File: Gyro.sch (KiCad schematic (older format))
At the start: 7 parts, among them U5 SN74AXC4T774BQBR, U6 ICM-20948

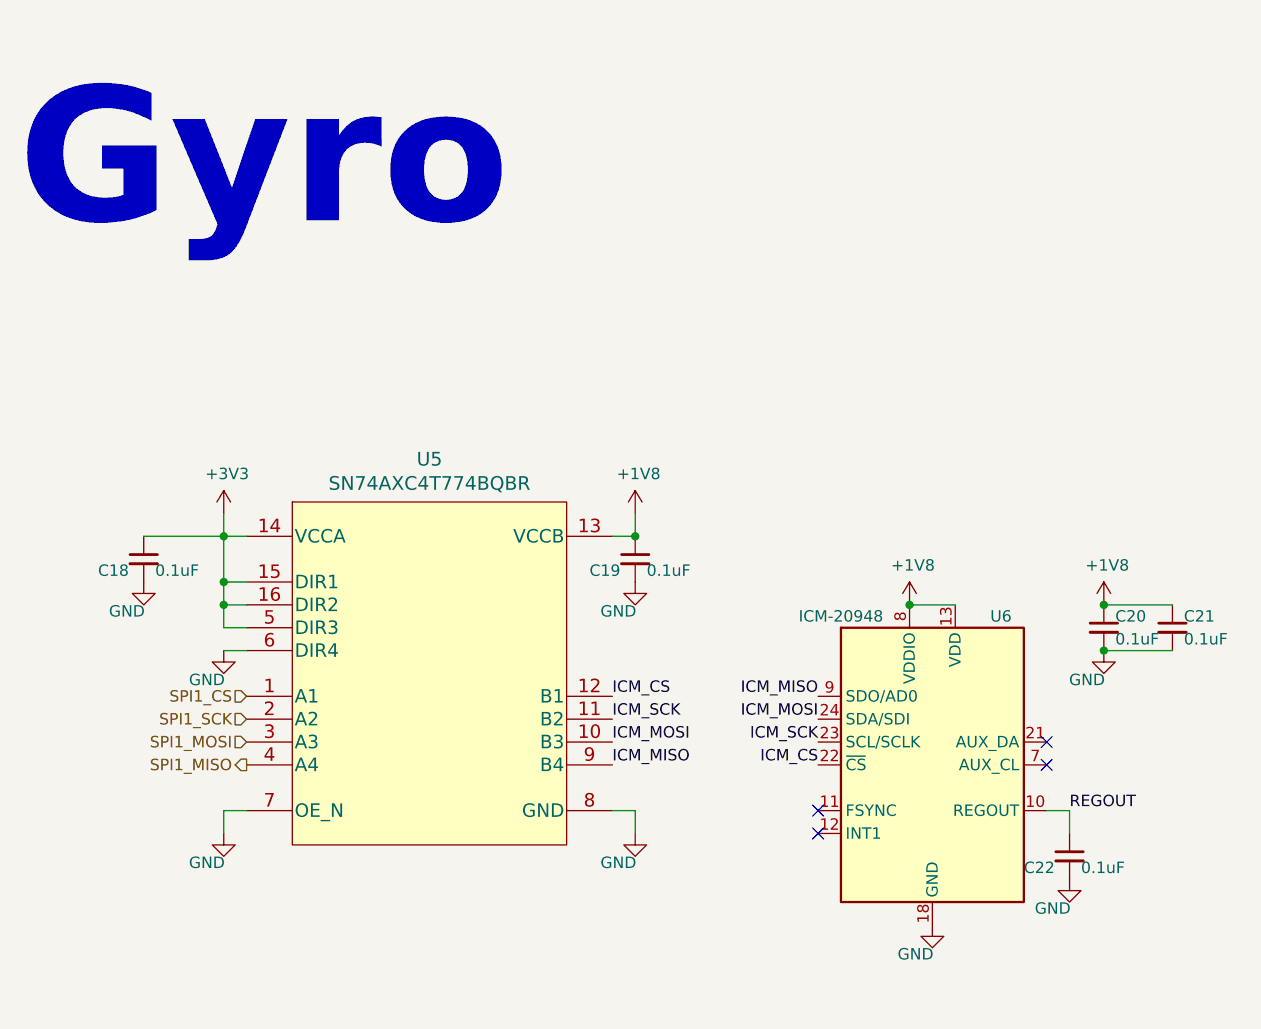
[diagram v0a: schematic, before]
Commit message: Changes made
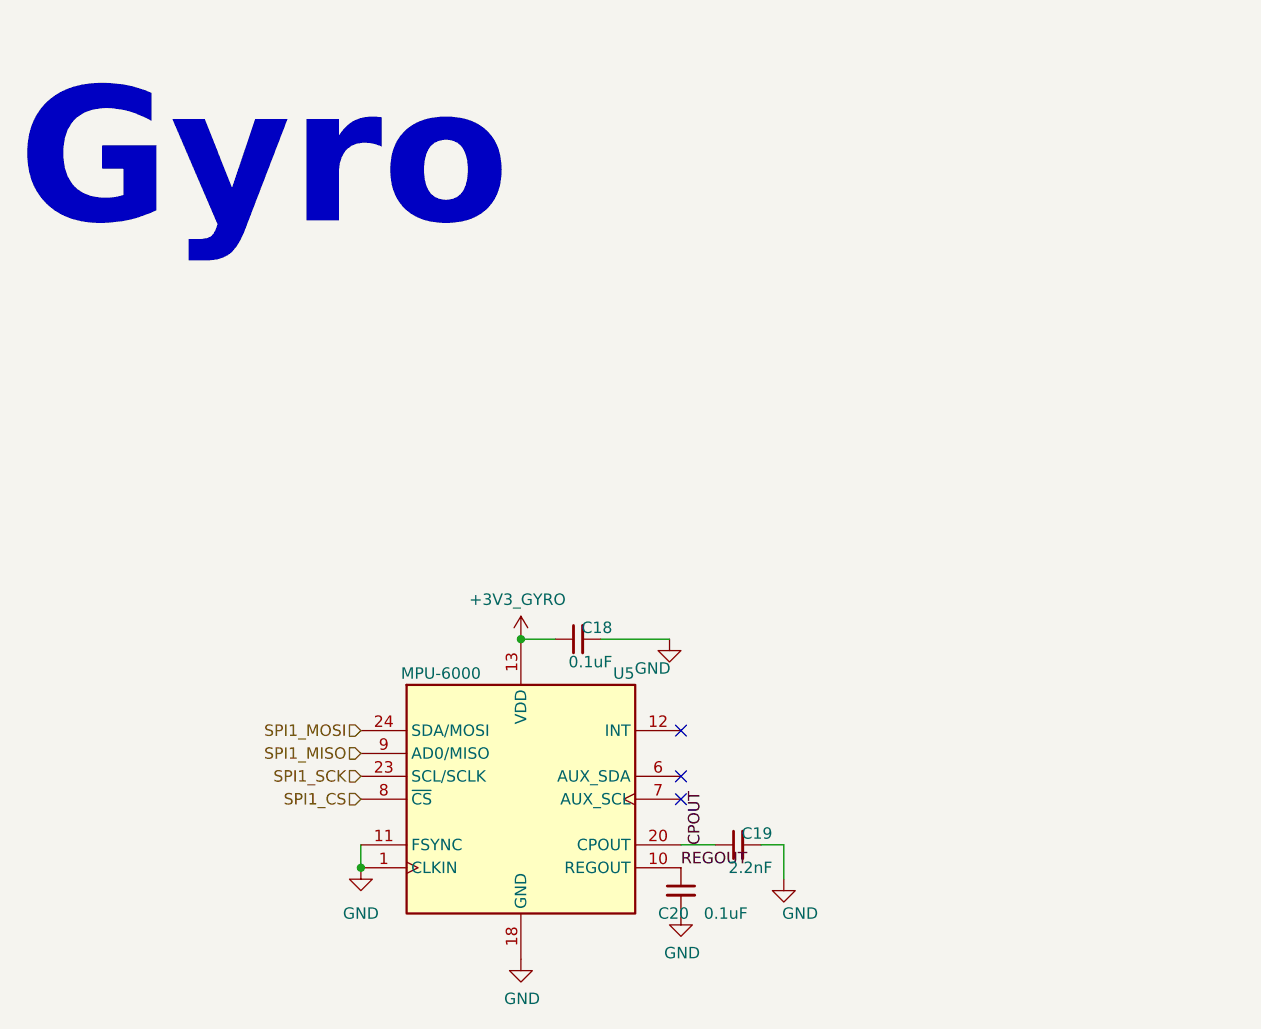
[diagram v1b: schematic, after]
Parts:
- removed C20, C21, C22: 0.1uF, Capacitor_SMD:C_0402_1005Metric, symbol Device:C_Small
- removed U5: SN74AXC4T774BQBR, Footprints:SN74AXC4T774BQBR, symbol JPW_Symbols:SN74AXC4T774BQBR
- removed U6: ICM-20948, Sensor_Motion:InvenSense_QFN-24_3x3mm_P0.4mm, symbol Sensor_Motion:ICM-20948
- added C18: 0.1uF, Capacitor_SMD:C_0402_1005Metric, symbol Device:C_Small
- added U5: MPU-6000, Sensor_Motion:InvenSense_QFN-24_4x4mm_P0.5mm, symbol Sensor_Motion:MPU-6000
- C19: value 0.1uF -> 2.2nF
- renumbered C18 to C20
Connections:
- net +3V3 is gone; now on net REGOUT: C20.1
- net GND: now also C18.2, U5.1 (CLKIN), U5.11 (FSYNC), U5.18 (GND)
- net REGOUT: now also U5.10 (REGOUT)
- net SPI1_CS: now also U5.8 (~CS)
- net SPI1_MISO: now also U5.9 (AD0/MISO)
- net SPI1_MOSI: now also U5.24 (SDA/MOSI)
- net SPI1_SCK: now also U5.23 (SCL/SCLK)
- net +1V8 renamed CPOUT
- net CPOUT: now also U5.20 (CPOUT)
- new net +3V3_GYRO: C18.1, U5.13 (VDD)
- no-connect marks 4 -> 3
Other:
- moved on the sheet: C20
